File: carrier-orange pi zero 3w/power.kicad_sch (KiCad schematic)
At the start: 22 parts, among them J4 Conn_01x04_Pin, J5 ORANGE_PI_POWER_CABLE, J6 5V_PERIPHERALS, U1 TPS54302DDCT

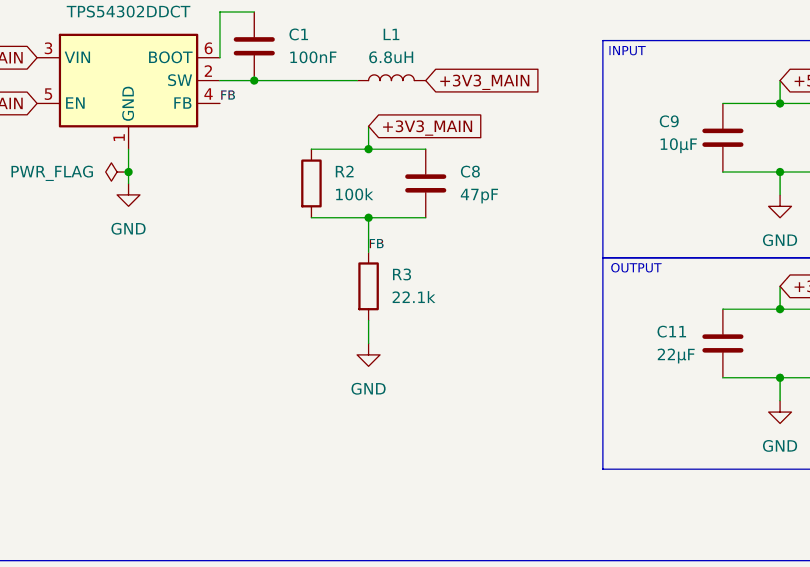
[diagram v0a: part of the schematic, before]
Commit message: ain
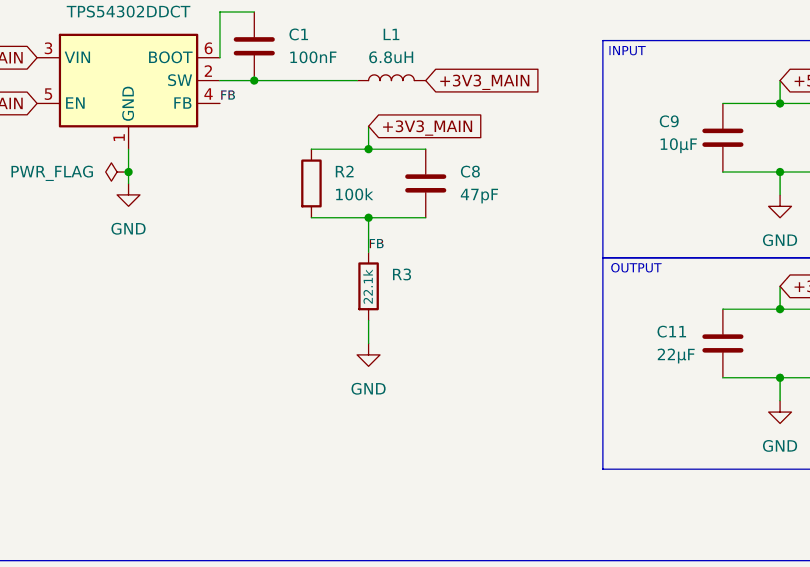
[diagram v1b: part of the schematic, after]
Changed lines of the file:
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@@
 		(in_pos_files yes)
 		(dnp no)
-		(fields_autoplaced yes)
 		(property "Reference" "R3"
 			(at 215.9 120.6499 0)
@@
 		)
 		(property "Value" "22.1k"
-			(at 215.9 123.1899 0)
+			(at 213.36 123.952 90)
 			(show_name no)
 			(do_not_autoplace no)
 			(effects
 				(font
-					(size 1.27 1.27)
+					(size 1.016 1.016)
 				)
 				(justify left)
